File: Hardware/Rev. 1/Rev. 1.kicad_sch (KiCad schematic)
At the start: 17 parts, among them J1 522711279, Q1 NMOS, U1 MCP73831-2-OT, U3 W25Q128JVS

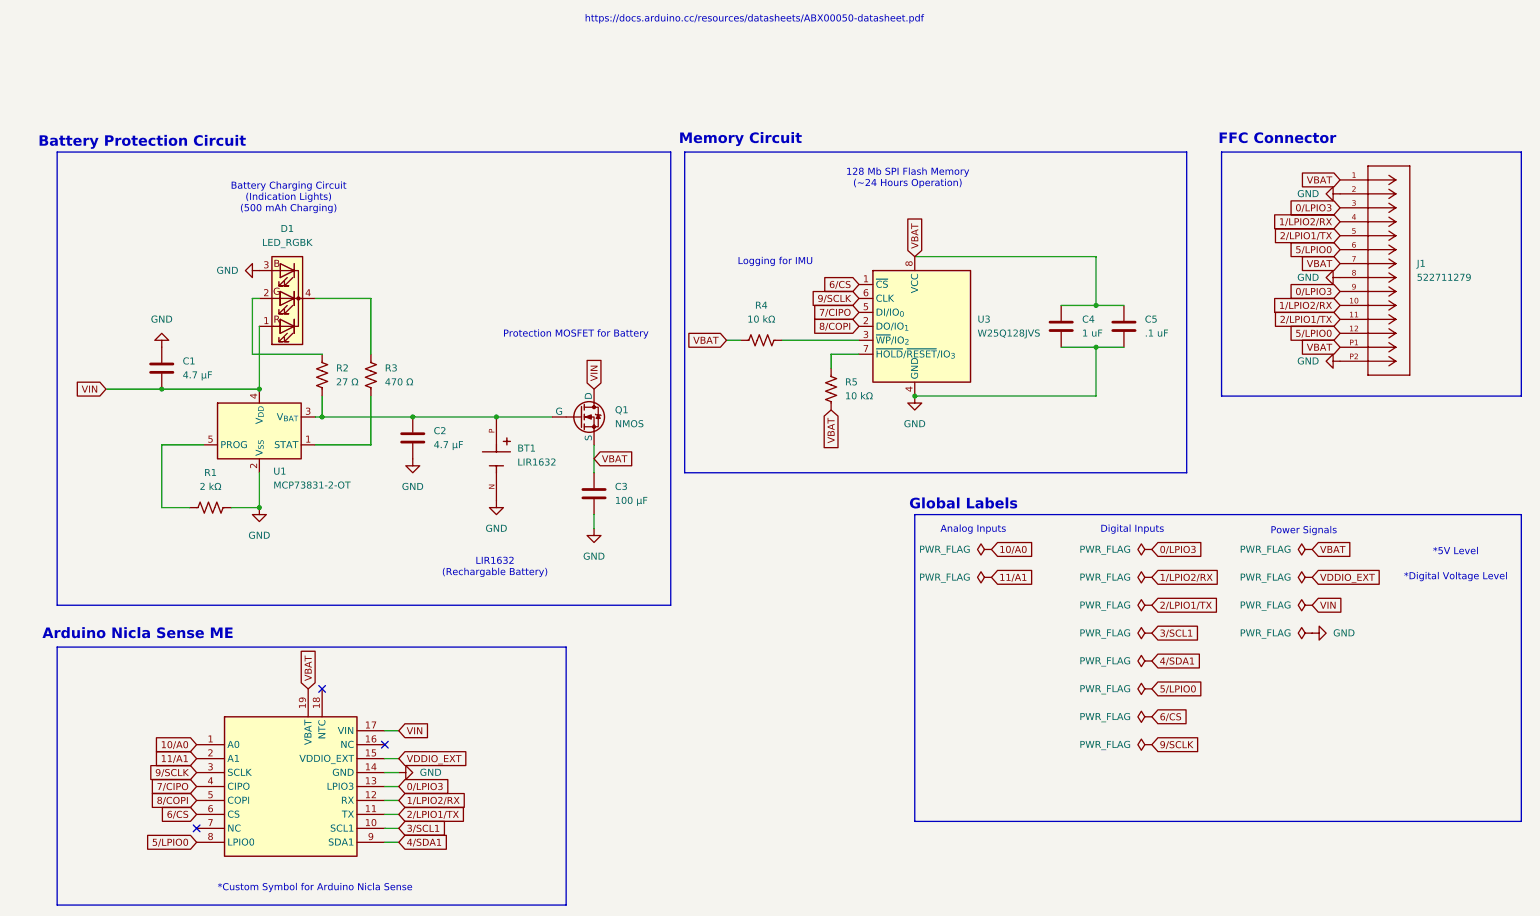
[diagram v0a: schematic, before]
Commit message: Hardware Changes
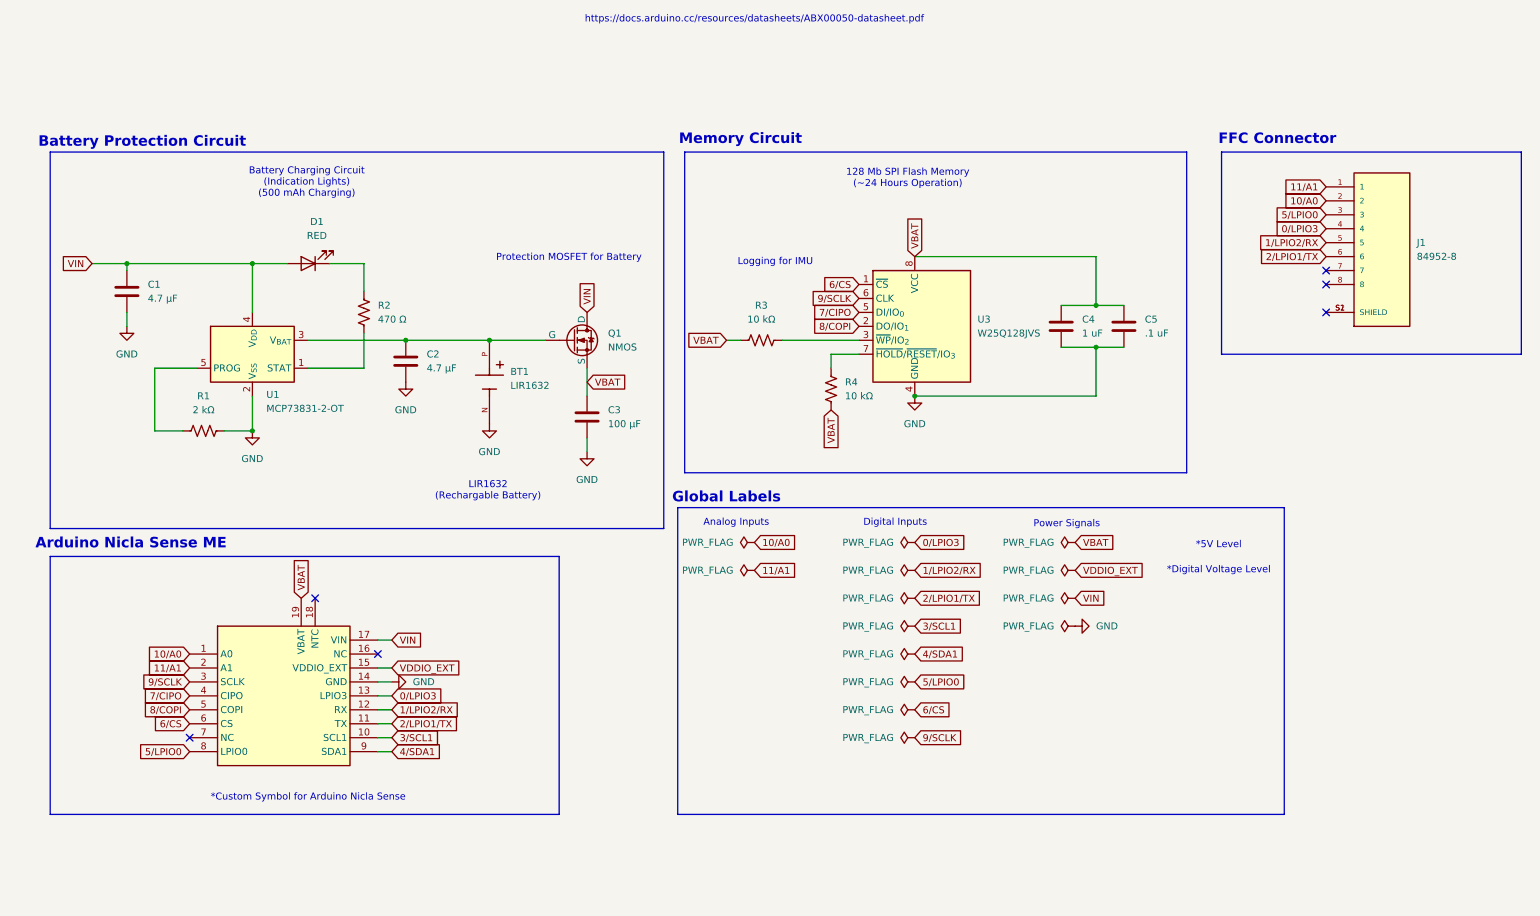
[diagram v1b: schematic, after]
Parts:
- removed D1: LED_RGBK, LED_SMD:LED_Kingbright_APFA3010_3x1.5mm_Horizontal, symbol Device:LED_RGBK
- removed J1: 522711279, footprints:FFC_522711279, symbol symbols:522711279
- removed R2: 27 Ω, Resistor_SMD:R_0201_0603Metric, symbol Device:R_US
- added D1: RED, Diode_SMD:D_0201_0603Metric, symbol Device:LED
- added J1: 84952-8, footprints:FFC_84952-8, symbol symbols:84952-8
- renumbered R3 to R2, R4 to R3, R5 to R4
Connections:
- net 0/LPIO3: now also J1.4
- net 10/A0: now also J1.2
- net 11/A1: now also J1.1
- net 1/LPIO2/RX: now also J1.5
- net 2/LPIO1/TX: now also J1.6
- net 5/LPIO0: now also J1.3
- net GND: now also C1.1; no longer C1.2
- net VIN: now also C1.2, D1.2 (A); no longer C1.1
- net at R2.1: now also D1.1 (K)
- new net: J1.S1 (SHIELD), J1.S2 (SHIELD)
- no-connect marks 3 -> 6
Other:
- moved on the sheet: BT1, C1, C2, C3, Q1, R1, R2, U1
